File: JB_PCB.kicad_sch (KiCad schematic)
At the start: 18 parts, among them J1 Conn_01x03_Pin, J10 Conn_01x03_Pin, J12 Conn_01x05_Pin, J2 Screw_Terminal_01x02, J3 Screw_Terminal_01x02, J4 Screw_Terminal_01x02, J5 Conn_01x03_Pin, J6 Screw_Terminal_01x02, J7 Conn_01x03_Pin, J8 Conn_01x03_Pin, J9 Conn_01x03_Pin

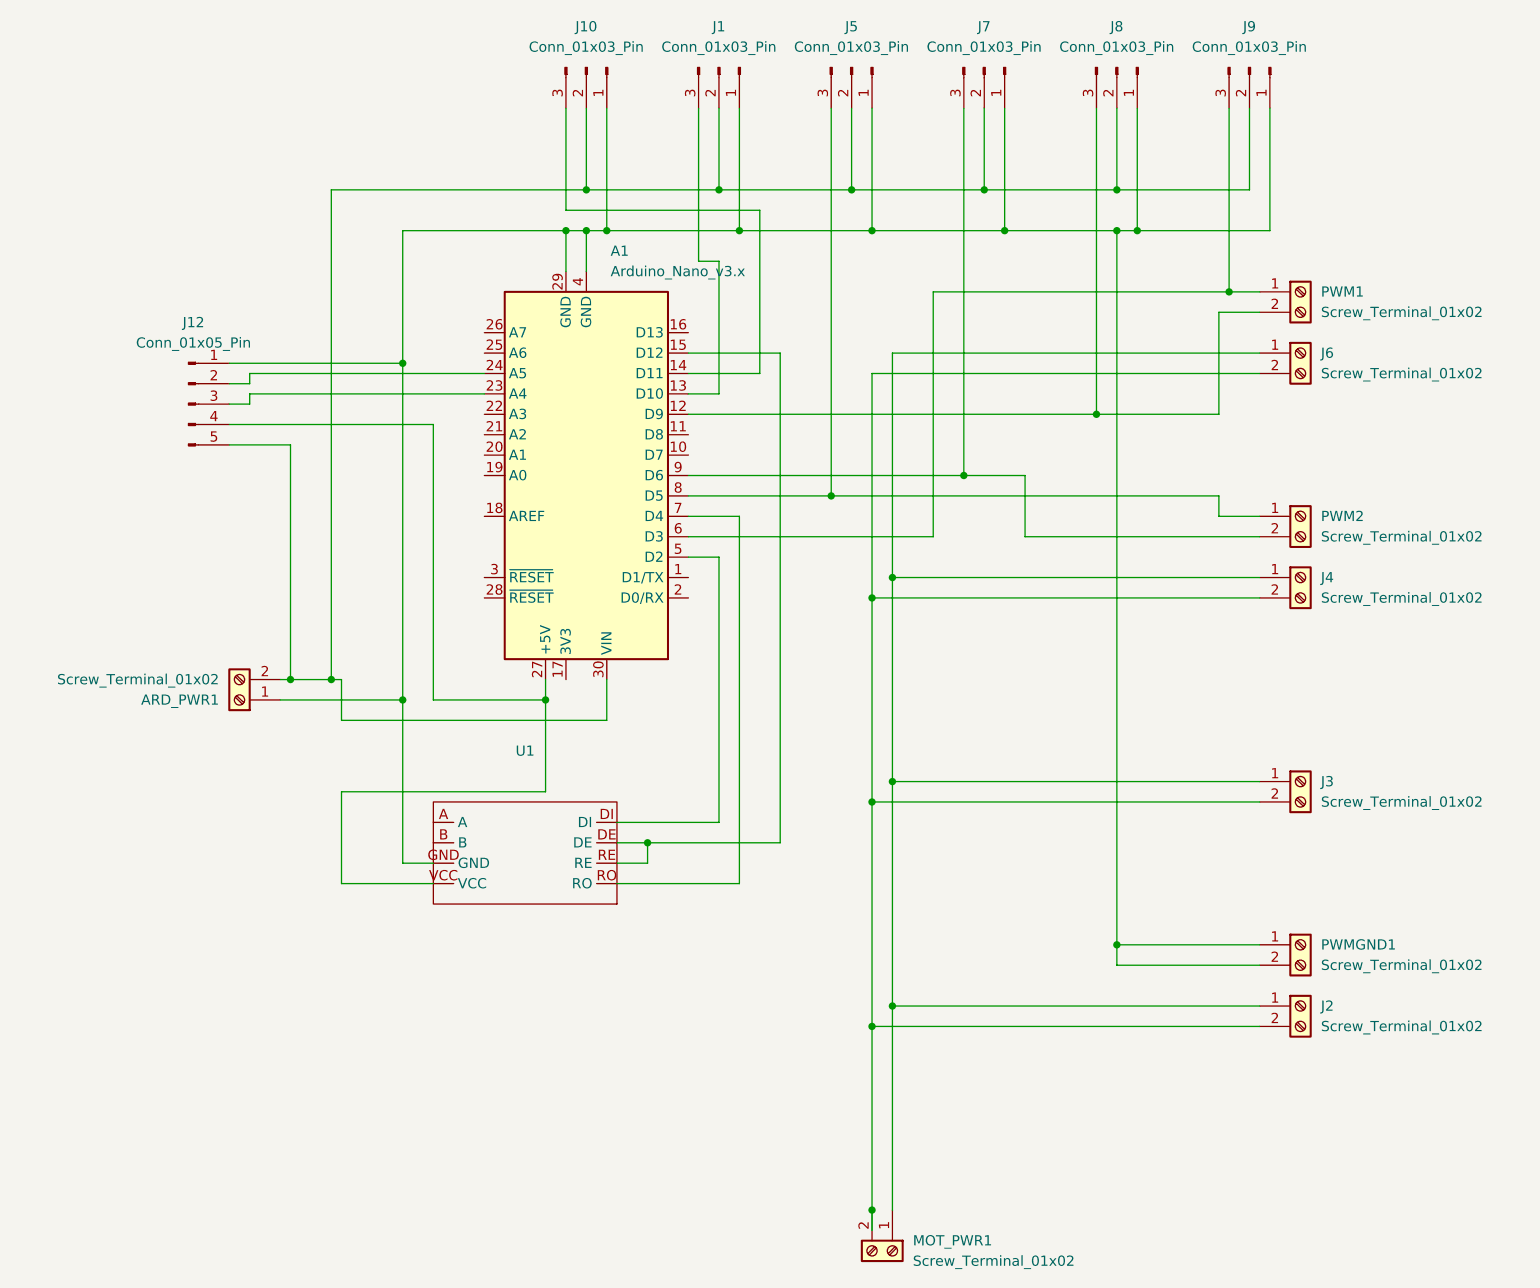
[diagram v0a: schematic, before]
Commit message: changes from my laptop from last year
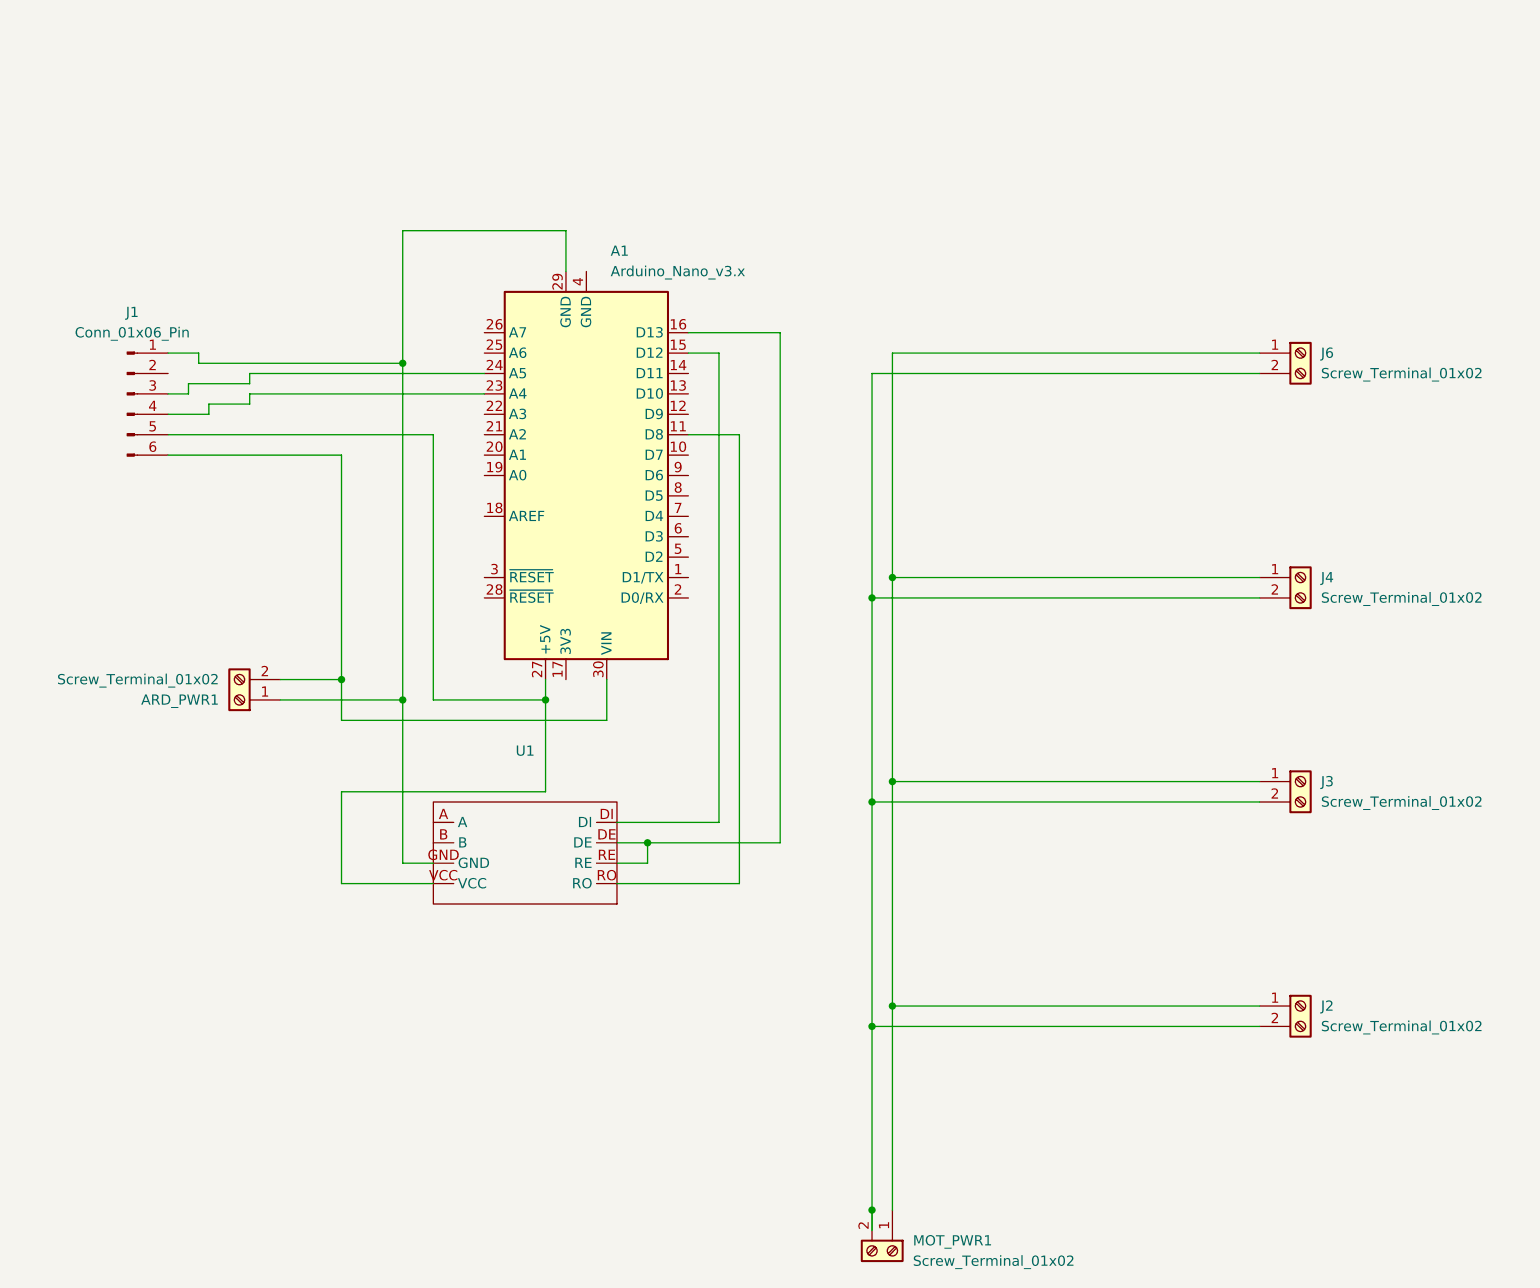
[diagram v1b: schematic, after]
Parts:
- removed J1, J10, J5, J7, J8, J9: Conn_01x03_Pin, myFootprints.pretty-master:3x1_Pin_Header, symbol Connector:Conn_01x03_Pin
- removed J12: Conn_01x05_Pin, myFootprints.pretty-master:1x5conn, symbol Connector:Conn_01x05_Pin
- removed PWM1, PWM2, PWMGND1: Screw_Terminal_01x02, myFootprints.pretty-master:screw 2x2, symbol Connector:Screw_Terminal_01x02
- added J1: Conn_01x06_Pin, myFootprints.pretty-master:1x6Headers, symbol Connector:Conn_01x06_Pin
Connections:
- net at A1.29 (GND), ARD_PWR1.1 (Pin_1), U1.GND: now also J1.1 (Pin_1); no longer A1.4 (GND)
- net at A1.30 (VIN), ARD_PWR1.2 (Pin_2): now also J1.6 (Pin_6)
- net at U1.DE, U1.RE: now also A1.16 (D13); no longer A1.15 (D12)
- net at U1.DI: now also A1.15 (D12); no longer A1.5 (D2)
- net at U1.RO: now also A1.11 (D8); no longer A1.7 (D4)
- net at A1.27 (+5V), U1.VCC: now also J1.5 (Pin_5)
- net at A1.24 (A5): now also J1.3 (Pin_3)
- net at A1.23 (A4): now also J1.4 (Pin_4)
